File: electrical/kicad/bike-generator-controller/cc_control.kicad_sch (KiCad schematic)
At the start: 7 parts, among them J1 J_CC_CTRL, U3 MCP4151-104E/SN

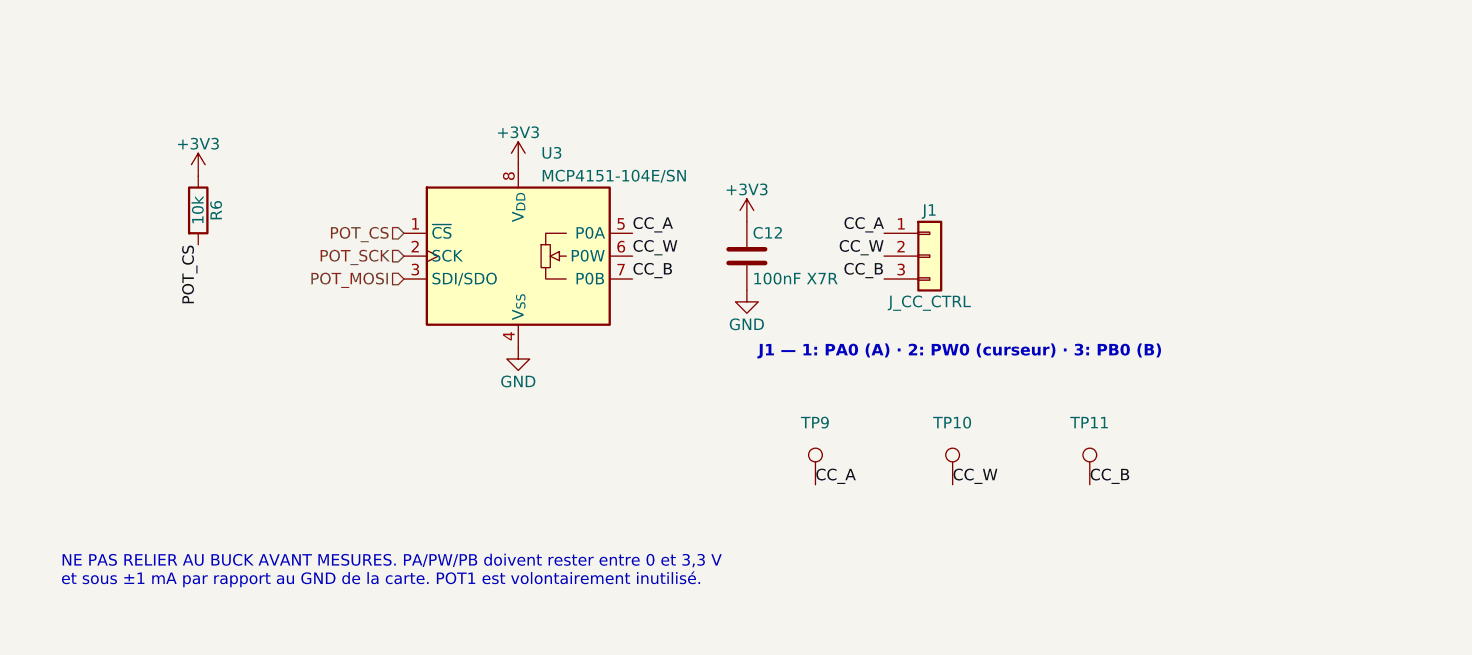
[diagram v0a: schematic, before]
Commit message: wip: checkpoint controller routing before review
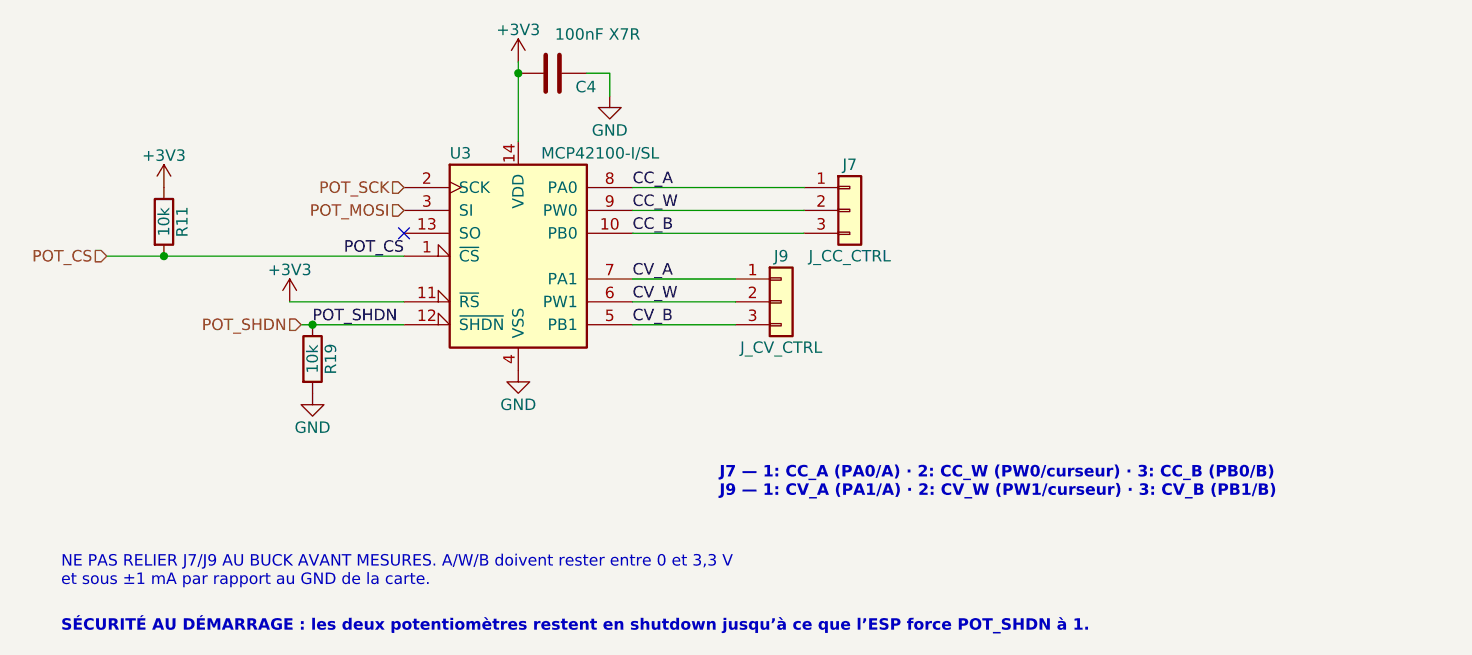
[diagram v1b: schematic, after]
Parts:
- removed TP10: CC_W, TestPoint:TestPoint_Pad_D1.5mm, symbol Connector:TestPoint
- removed TP11: CC_B, TestPoint:TestPoint_Pad_D1.5mm, symbol Connector:TestPoint
- removed TP9: CC_A, TestPoint:TestPoint_Pad_D1.5mm, symbol Connector:TestPoint
- removed U3: MCP4151-104E/SN, Package_SO:SOIC-8_3.9x4.9mm_P1.27mm, symbol Potentiometer_Digital:MCP4151-xxxx-P
- added J9: J_CV_CTRL, Connector_PinHeader_2.54mm:PinHeader_1x03_P2.54mm_Vertical, symbol Connector_Generic:Conn_01x03
- added R19: 10k, Resistor_SMD:R_0805_2012Metric_Pad1.20x1.40mm_HandSolder, symbol Device:R
- added U3: MCP42100-I/SL, Package_SO:SOIC-14_3.9x8.7mm_P1.27mm, symbol Potentiometer_Digital:MCP42100
- renumbered C12 to C4, J1 to J7, R6 to R11
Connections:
- net +3V3: now also C4.2, U3.11 (~{RS}), U3.14 (VDD); no longer C4.1
- net CC_A: now also U3.8 (PA0)
- net CC_B: now also U3.10 (PB0)
- net CC_W: now also U3.9 (PW0)
- net GND: now also C4.1, R19.2, U3.4 (VSS); no longer C4.2
- net POT_CS: now also U3.1 (~{CS})
- net POT_MOSI: now also U3.3 (SI)
- net POT_SCK: now also U3.2 (SCK)
- new net CV_A: J9.1 (Pin_1), U3.7 (PA1)
- new net CV_B: J9.3 (Pin_3), U3.5 (PB1)
- new net CV_W: J9.2 (Pin_2), U3.6 (PW1)
- new net POT_SHDN: R19.1, U3.12 (~{SHDN})
- no-connect marks 0 -> 1
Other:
- note added: "J7 — 1: CC_A (PA0/A) · 2: CC_W (PW0/curseur) · 3: CC_B (PB0/B) J9 — 1: CV_A (PA1/A) · 2: CV_W (PW1/curseur) · 3: CV_B (PB1/B)"
- note added: "NE PAS RELIER J7/J9 AU BUCK AVANT MESURES. A/W/B doivent rester entre 0 et 3,3 V et sous ±1 mA par rapport au GND de la carte."
- note added: "SÉCURITÉ AU DÉMARRAGE : les deux potentiomètres restent en shutdown jusqu’à ce que l’ESP force POT_SHDN à 1."
- note removed: "J1 — 1: PA0 (A) · 2: PW0 (curseur) · 3: PB0 (B)"
- note removed: "NE PAS RELIER AU BUCK AVANT MESURES. PA/PW/PB doivent rester entre 0 et 3,3 V et sous ±1 mA par rapport au GND de la carte. POT1 est volontairement inutilisé."
- moved on the sheet: C4, J7, R11
